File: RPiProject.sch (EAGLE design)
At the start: 18 parts, among them M1 MOTOR10MM, M2 MOTOR10MM

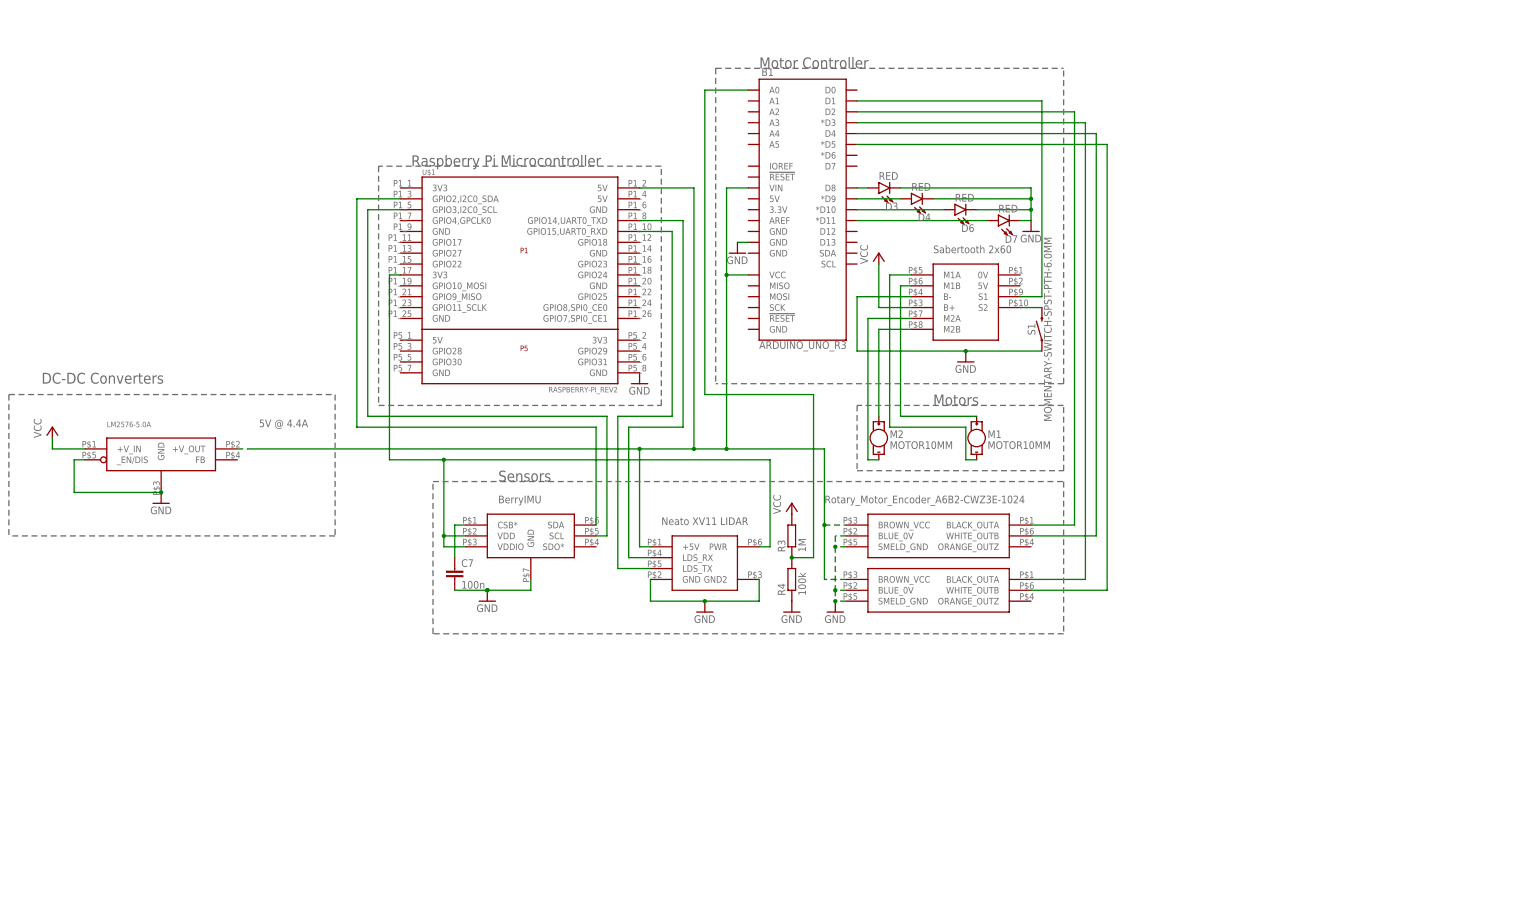
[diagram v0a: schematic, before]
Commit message: Version 7
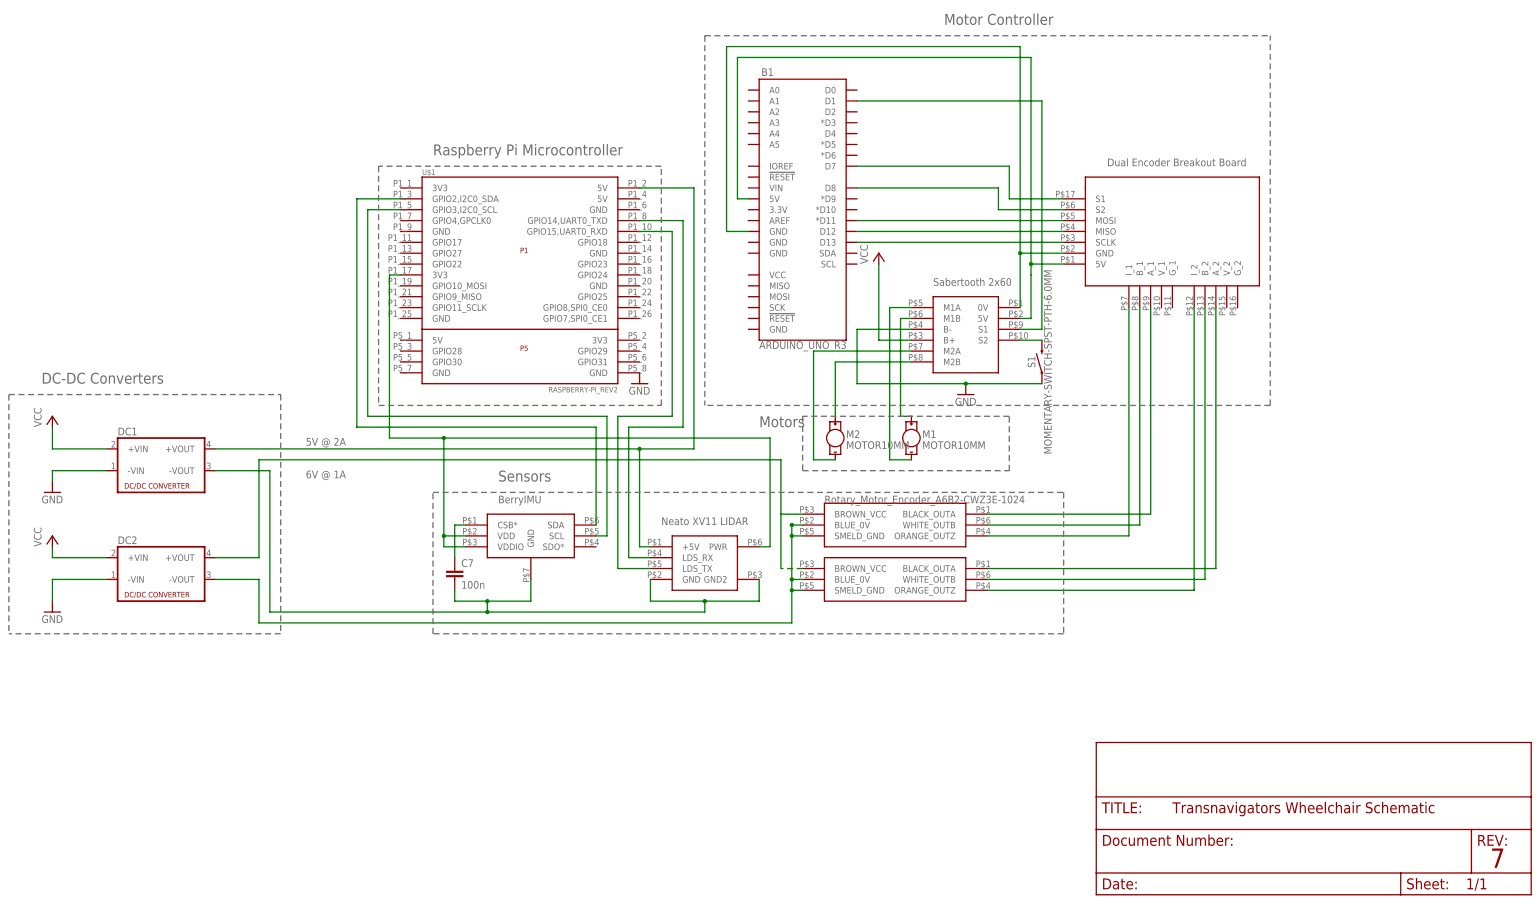
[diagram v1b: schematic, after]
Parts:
- removed D3, D4, D6, D7: RED, SparkFun-LED:LED-RED0603
- removed LM2576-5.0A: (no value), LM2576:LM2576-T05A
- removed R3: 1M, ee2parts:R
- removed R4: 100k, ee2parts:R
- added DC1, DC2: (no value), dc-dc-converter:NME
- added U$5: DUAL_LS7366R, RaspberryPi:DUAL_LS7366R
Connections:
- removed net GND2: LM2576-5.0A.GND, LM2576-5.0A._EN/DIS
- new net N$14: B1.5V, U$5.5V, U$6.5V
- new net N$16: B1.GND@2, U$5.GND, U$6.0V
- new net N$18: C7.2, DC1.-VOUT, U$4.GND, XV11LIDAR.GND, XV11LIDAR.GND2
- new net N$20: DC2.-VOUT, U$2.BLUE_0V, U$2.SMELD_GND, U$3.BLUE_0V, U$3.SMELD_GND
- new net N$23: B1.D13, U$5.SCLK
- new net N$24: U$2.ORANGE_OUTZ, U$5.I_1
- new net N$25: U$3.ORANGE_OUTZ, U$5.I_2
- net GND: now also DC1.-VIN, DC2.-VIN; no longer B1.GND@1, C7.2, R4.1, U$2.BLUE_0V, U$2.SMELD_GND, U$3.BLUE_0V, U$3.SMELD_GND, U$4.GND, XV11LIDAR.GND, XV11LIDAR.GND2
- net N$11: now also U$5.A_1; no longer B1.D2
- net N$19: now also U$5.A_2; no longer B1.*D3
- net N$2: now also DC1.+VOUT; no longer B1.VCC, B1.VIN, LM2576-5.0A.+V_OUT, U$2.BROWN_VCC, U$3.BROWN_VCC
- net N$21: now also U$5.B_2; no longer B1.*D5
- net N$22: now also U$5.B_1; no longer B1.D4
- net N$27: now also B1.D12, U$5.MISO; no longer B1.*D9, D4.A
- net N$28: now also B1.*D11, U$5.MOSI; no longer B1.*D10, D6.A
- net N$29: now also B1.D7, U$5.S1; no longer B1.*D11, D7.A
- net N$30: now also B1.D8, U$5.S2; no longer D3.C, D4.C, D6.C, D7.C
- net N$4: now also U$2.BROWN_VCC; no longer B1.A0, R3.1, R4.2
- net N$9: now also DC2.+VOUT, U$3.BROWN_VCC; no longer B1.D8, D3.A
- net VCC: now also DC1.+VIN, DC2.+VIN; no longer LM2576-5.0A.+V_IN, R3.2
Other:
- note added: "5V @ 2A"
- note added: "6V @ 1A"
- note added: "Dual Encoder Breakout Board"
- note removed: "5V @ 4.4A"
- moved on the sheet: M1, M2, S1

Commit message: i2c and dc-dc converter changes
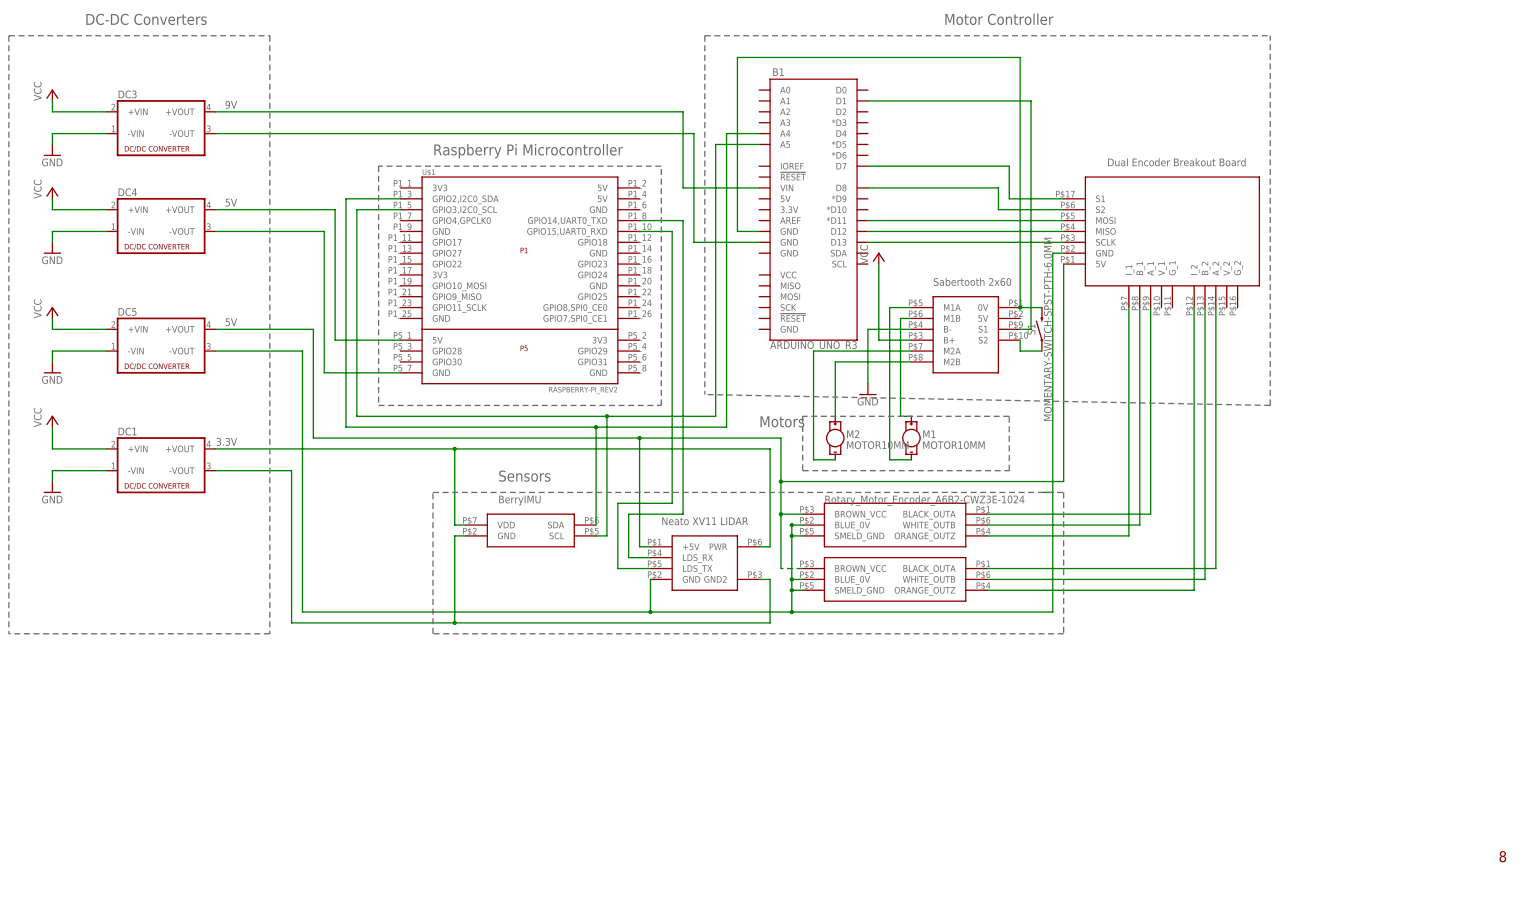
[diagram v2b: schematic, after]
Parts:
- removed C7: 100n, ee2parts:C2.5P
- removed DC2: (no value), dc-dc-converter:NME
- added DC3, DC4, DC5: (no value), dc-dc-converter:NME
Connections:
- removed net N$14: B1.5V, U$5.5V, U$6.5V
- removed net N$18: C7.2, DC1.-VOUT, U$4.GND, XV11LIDAR.GND, XV11LIDAR.GND2
- removed net N$2: DC1.+VOUT, U$1.5V@2, XV11LIDAR.+5V
- removed net N$20: DC2.-VOUT, U$2.BLUE_0V, U$2.SMELD_GND, U$3.BLUE_0V, U$3.SMELD_GND
- new net N$31: B1.VIN, DC3.+VOUT
- new net N$32: B1.A4, U$1.GPIO2,I2C0_SDA, U$4.SDA
- new net N$33: DC4.+VOUT, U$1.5V@P5_1
- new net N$34: DC4.-VOUT, U$1.GND@P5_7
- net GND: now also DC3.-VIN, DC4.-VIN, DC5.-VIN; no longer DC2.-VIN, S1.1, U$1.GND@P5_8
- net N$12: now also B1.A5
- net N$15: now also S1.1, U$6.S2; no longer U$1.GPIO2,I2C0_SDA, U$4.SDA
- net N$16: now also S1.2; no longer U$5.GND
- net N$17: now also B1.GND@1, DC3.-VOUT; no longer S1.2, U$6.S2
- net N$4: now also DC5.-VOUT, U$2.BLUE_0V, U$2.SMELD_GND, U$3.BLUE_0V, U$3.SMELD_GND, U$5.GND, XV11LIDAR.GND; no longer U$2.BROWN_VCC
- net N$5: now also DC1.+VOUT; no longer U$1.3V3@17, U$4.VDDIO
- net N$6: now also DC5.+VOUT, U$2.BROWN_VCC, U$3.BROWN_VCC, U$5.5V, XV11LIDAR.+5V; no longer C7.1, U$4.CSB*
- net N$9: now also DC1.-VOUT, U$4.GND, XV11LIDAR.GND2; no longer DC2.+VOUT, U$3.BROWN_VCC
- net VCC: now also DC3.+VIN, DC4.+VIN, DC5.+VIN; no longer DC2.+VIN
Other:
- note added: "3.3V"
- note added: "5V"
- note added: "8"
- note added: "9V"
- note removed: "5V @ 2A"
- note removed: "6V @ 1A"
- moved on the sheet: B1, S1
